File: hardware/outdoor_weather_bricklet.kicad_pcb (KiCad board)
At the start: 2 copper layers, 45 x 25 mm, 36 parts, among them J1 Debug, P1 CON-SENSOR2, P2 Boot, U1 XMC1XXX24, U2 MCP4018, U3 AM612, U4 DRILL, U5 DRILL, U6 DRILL, U7 DRILL

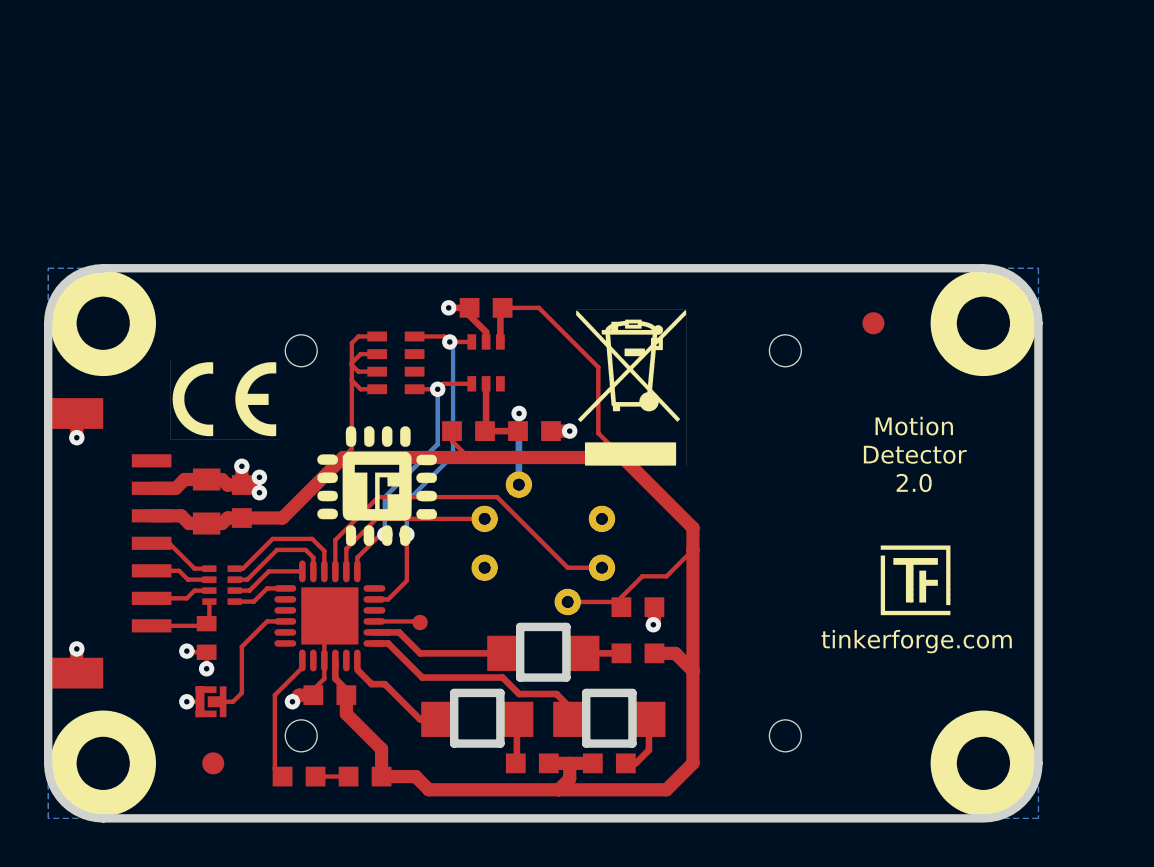
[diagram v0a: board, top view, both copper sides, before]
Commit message: briklet finished
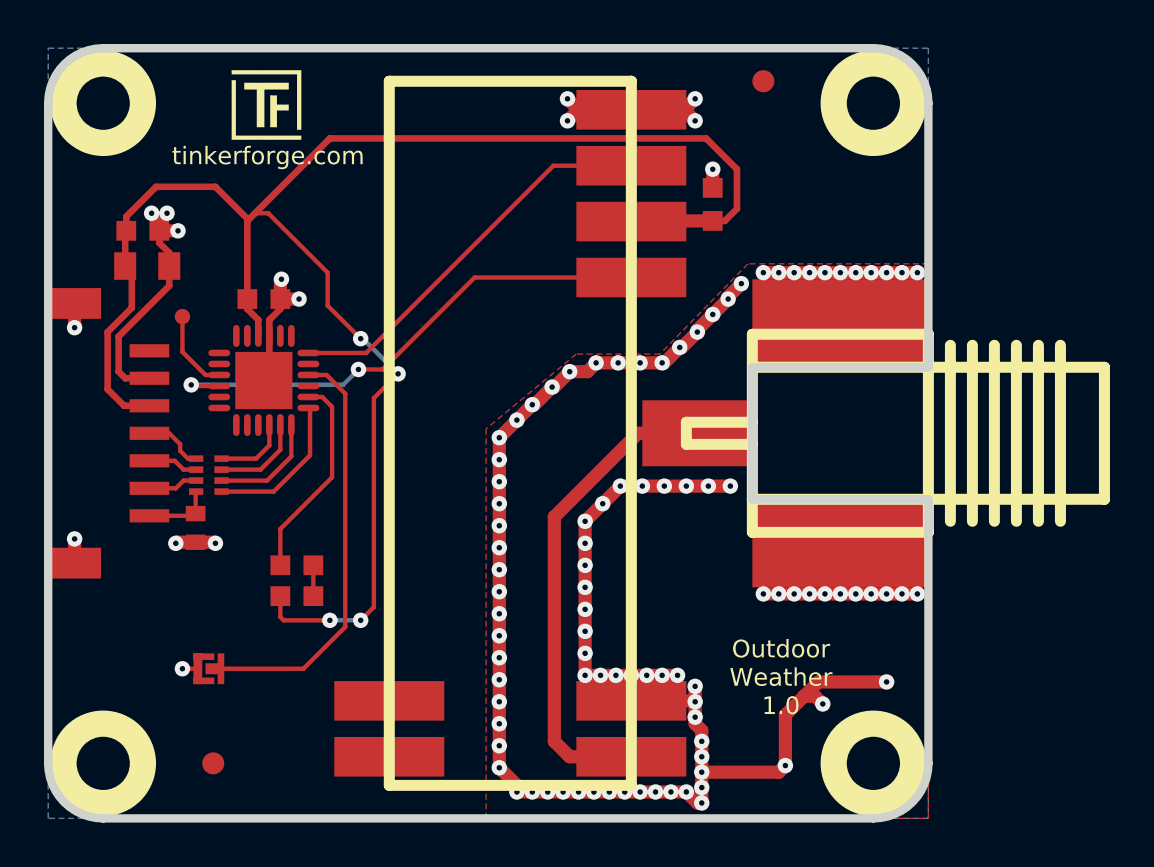
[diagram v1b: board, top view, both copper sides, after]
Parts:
- removed C6, C7: 100nF, C0603F
- removed D2: red_inv, D1206_INV
- removed D3: green_inv, D1206_INV
- removed D4: blue_inv, D1206_INV
- removed the G*** at (84.1, 39.4)
- removed R2: 30k, R0603F
- removed R3, R4: 68, R0603F
- removed R5: 22, R0603F
- removed REF**: Fresnel_Lens_S8002, kicad-libraries:Fresnel_Lens_S8002
- removed RP2: 4k7, kicad-libraries:4X0603
- removed U3: AM612, AM612
- removed the VAL at (69.4, 35.2)
- removed the VAL at (51.0, 35.8)
- added ANT1: FT-004B, FT-004B, F.Cu at (82.9, 37.3)
- added VAL: WEEE_7mm, kicad-libraries:WEEE_7mm, B.Cu at (62.9, 27.3)
- added VAL: CE_5mm, kicad-libraries:CE_5mm, B.Cu at (62.9, 47.3)
- G***: moved to B.Cu
- U2: value MCP4018 -> RFM210LCF-S1; footprint kicad-libraries:SC70-6 -> RFM210LCF-S1
- U4, U5, U6, U7: footprint kicad-libraries:DRILL_NP -> DRILL_NP
- moved G*** 36.6 mm to (54.4, 20.8)
- moved C4 18.2 mm to (52.7, 31.2), turned to 180 degrees
- moved J1 17.6 mm to (49.0, 32.0)
- moved C5 13.1 mm to (73.1, 26.9), turned to 270 degrees
- moved C3 13.1 mm to (47.2, 28.1), turned to 180 degrees
- moved Fiducial_Mark 12.1 mm to (75.4, 21.3)
- moved U7 11.2 mm to (80.4, 22.3)
- moved U1 11.1 mm to (52.7, 34.9), turned to 180 degrees
- moved C2 11.0 mm to (47.4, 29.7), turned to 180 degrees
- moved U6 10.00 mm to (45.4, 22.3)
- moved R1 9.60 mm to (54.2, 43.3)
- moved D1 8.77 mm to (54.2, 44.7), turned to 0 degrees
- moved G*** 5.59 mm to (62.9, 37.3), turned to 180 degrees
- moved RP1 5.04 mm to (50.2, 39.2)
- moved C1 5.02 mm to (49.6, 41.6)
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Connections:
- C5 pad 2: VSENS -> VCC
- U1 pad 12: LED_BLUE -> (no net)
- U1 pad 13: LED_GREEN -> (no net)
- U1 pad 14: LED_RED -> (no net)
- U1 pad 16: (no net) -> SDN
- U1 pad 17: SCL -> (no net)
- U1 pad 19: SDA -> (no net)
- U1 pad 2: (no net) -> Net-(R1-Pad1)
- U1 pad 20: ENABLE -> (no net)
- U1 pad 21: VOUT -> (no net)
- U1 pad 6: (no net) -> DATA
- U1 pad 7: Net-(R1-Pad1) -> (no net)
- U2 pad 1: VCC -> Net-(ANT1-Pad1)
- U2 pad 3: SCL -> SDN
- U2 pad 4: SDA -> VCC
- U2 pad 5: VSENS -> DATA
- U2 pad 6: (no net) -> GND
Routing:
- net GND: track 25.6 -> 133.3 mm, vias 12 -> 110
- net SDN: track 0.00 -> 23.3 mm, vias 0 -> 2
- net Net-(ANT1-Pad1): track 0.00 -> 22.1 mm
- net DATA: track 0.00 -> 18.2 mm
- net SCL: track 16.3 -> 0.00 mm, vias 2 -> 0
- net VOUT: track 15.7 -> 0.00 mm
- net VCC: track 95.4 -> 81.0 mm, vias 0 -> 4
- net Net-(P2-Pad2): track 5.97 -> 19.6 mm
- net SDA: track 12.6 -> 0.00 mm, vias 2 -> 0
- net LED_GREEN: track 11.3 -> 0.00 mm
- net ENABLE: track 7.87 -> 0.00 mm
- net VSENS: track 7.79 -> 0.00 mm, vias 1 -> 0
- net LED_RED: track 6.27 -> 0.00 mm
- net LED_BLUE: track 5.01 -> 0.00 mm
- net S-MISO: track 2.55 -> 6.89 mm
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- added copper zone on F.Cu, net GND
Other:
- board size 45 x 25 mm -> 40 x 35 mm
- board text added: "Outdoor Weather 1.0"
- board text removed: "Motion Detector 2.0"
